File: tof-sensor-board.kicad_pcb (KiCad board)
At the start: 2 copper layers, 22.8 x 16.8 mm, 30 parts, among them U1 STM32F302K8U6, U2 LTC2875, U3 MCP1703, U4 VL53L0X, X1 16MHz

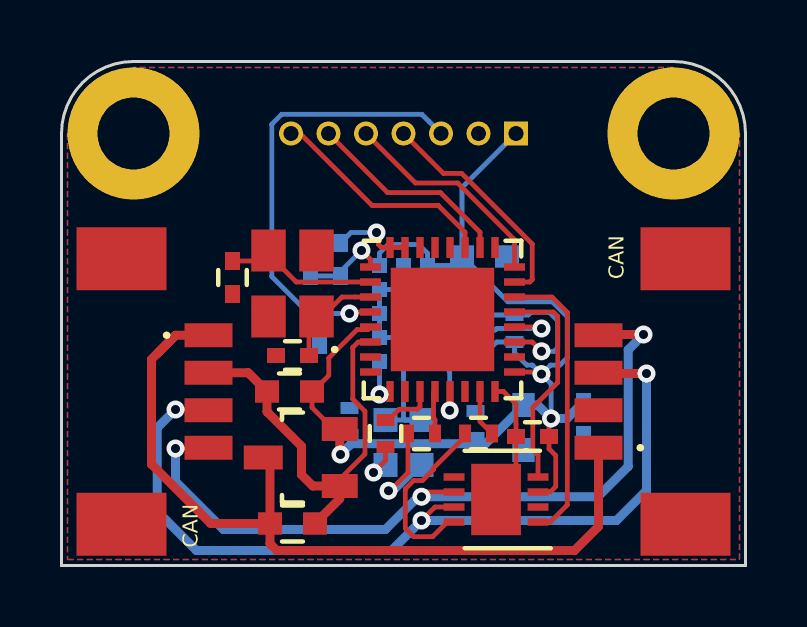
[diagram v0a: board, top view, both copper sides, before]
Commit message: routing finished
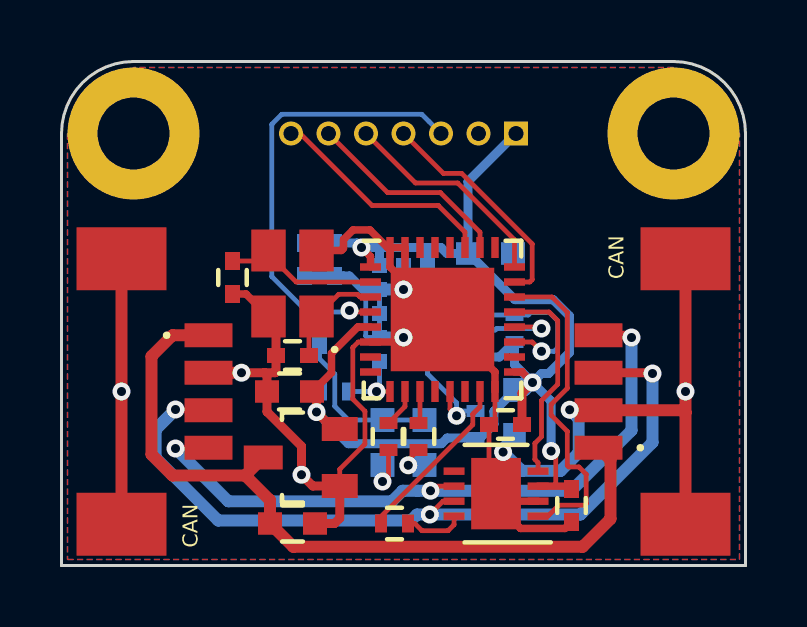
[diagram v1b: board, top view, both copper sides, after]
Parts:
- added G***: LOGO, _logo:CVRA-logo-small, B.Cu at (59.0, 56.0)
- C7: moved to F.Cu
- moved R8 4.10 mm to (49.7, 57.0), turned to 180 degrees
- moved C11 2.64 mm to (55.6, 56.4), turned to 270 degrees
- moved C7 2.61 mm to (53.4, 53.7), turned to 180 degrees
- moved R9 1.12 mm to (47.7, 52.6), turned to 0 degrees
- moved C1 0.58 mm to (53.7, 53.3)
- moved C14 0.22 mm to (52.9, 48.0)
- moved C13 0.20 mm to (46.7, 48.2), turned to 270 degrees
- moved C2 0.20 mm to (47.7, 48.2), turned to 270 degrees
- moved U2 0.20 mm to (53.1, 56.0)
- moved R6 0.14 mm to (49.5, 54.1)
- moved R7 0.14 mm to (50.5, 54.1), turned to 90 degrees
- moved D2 0.10 mm to (49.3, 54.3)
- moved D3 0.10 mm to (50.7, 54.3)
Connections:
- MEC1 pad 1: (no net) -> GND
- MEC2 pad 1: (no net) -> GND
- U1 pad 10: (no net) -> /Proximity
- U1 pad 11: /Proximity -> /Error
- U1 pad 12: /Error -> (no net)
- U1 pad 33: (no net) -> GND
- U2 pad 9: Net-(U2-Pad9) -> GND
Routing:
- net GND: track 28.1 -> 80.9 mm, vias 1 -> 8
- net /CAN_SPEED: track 1.57 -> 5.77 mm
- net Net-(R8-Pad1): track 6.10 -> 2.00 mm
- net Net-(CONN2-Pad4): track 26.1 -> 23.1 mm
- net Net-(D3-Pad2): track 3.66 -> 1.20 mm
- net VCC: track 42.7 -> 44.5 mm
- net Net-(CONN2-Pad3): track 29.2 -> 27.5 mm
- net Net-(U2-Pad9): track 1.61 -> 0.00 mm
- net /CAN_TX: track 9.60 -> 11.0 mm
- net +5V: track 28.3 -> 26.9 mm
- net /GPIO1: track 2.81 -> 3.81 mm
- net /XSHUT: track 1.56 -> 2.44 mm
- net /Proximity: track 1.84 -> 1.28 mm
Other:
- rule trace_min: 0.1524 -> 0.16
- board text added: "CVRA"
- board text added: "VL53L0X TOF Sensor RevA"
